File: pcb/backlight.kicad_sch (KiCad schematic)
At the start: 52 parts, among them U1 AL8860WT, U3 AL8860WT, U4 AL8860WT

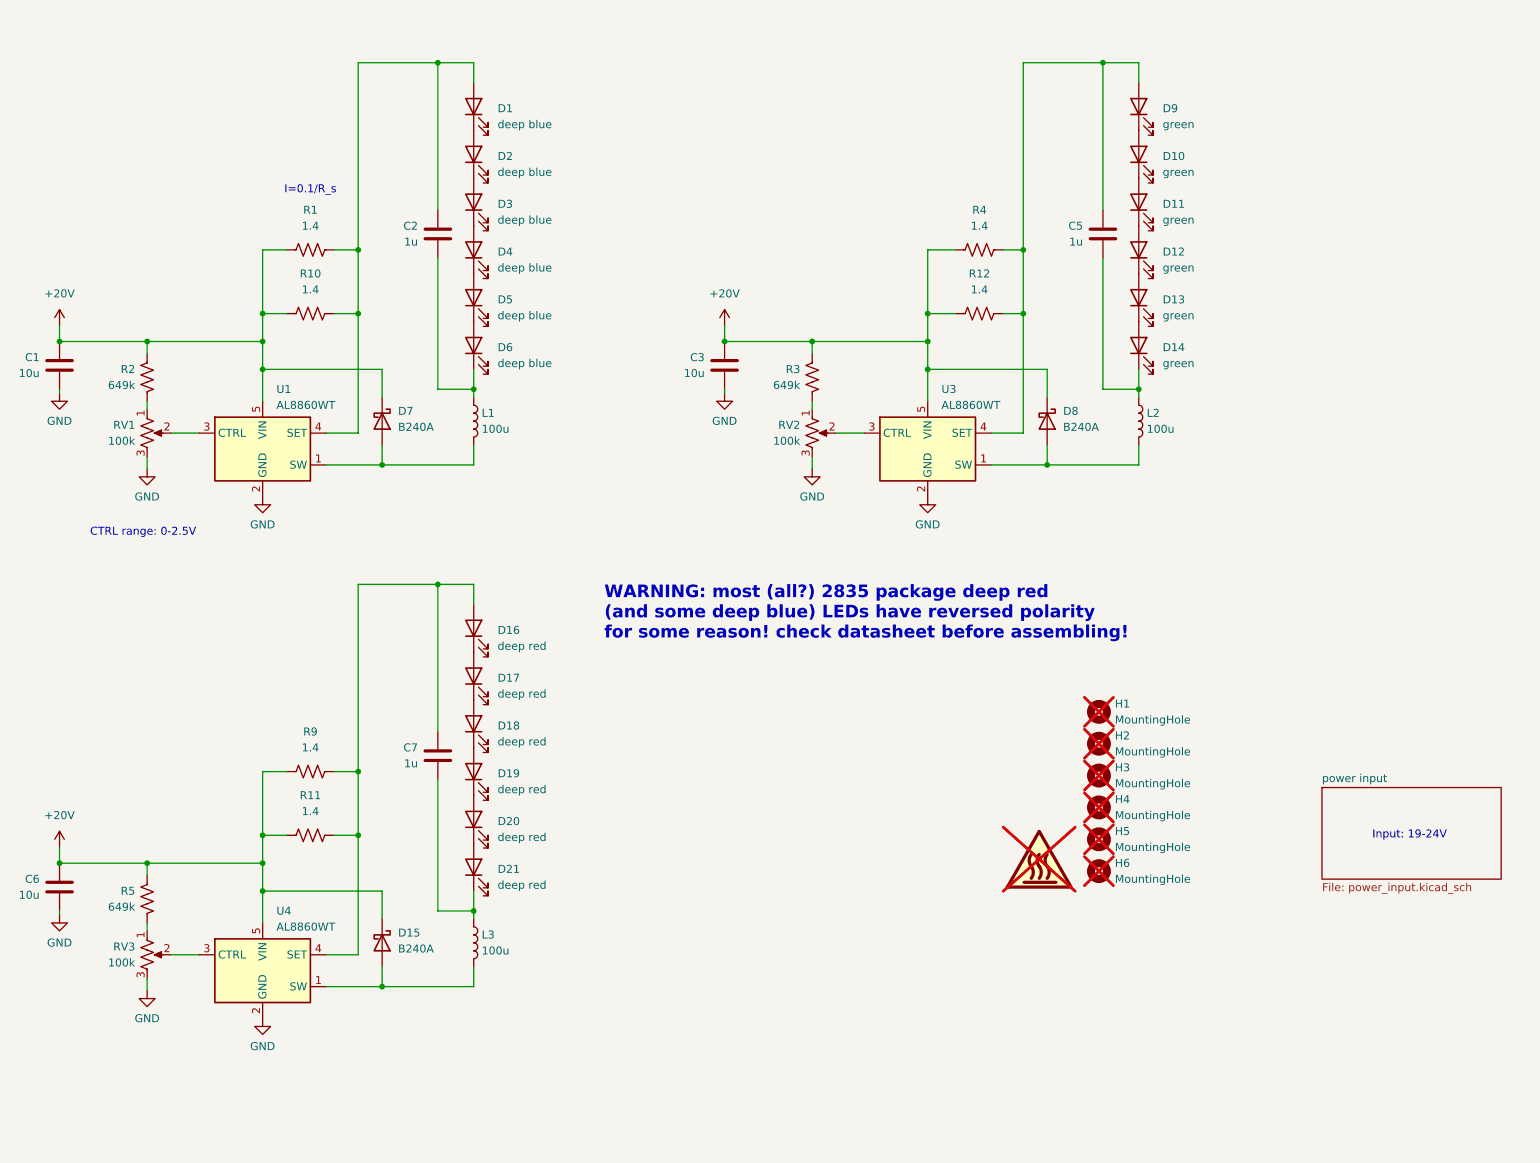
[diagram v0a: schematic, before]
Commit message: PCB for 4x5 scanlight
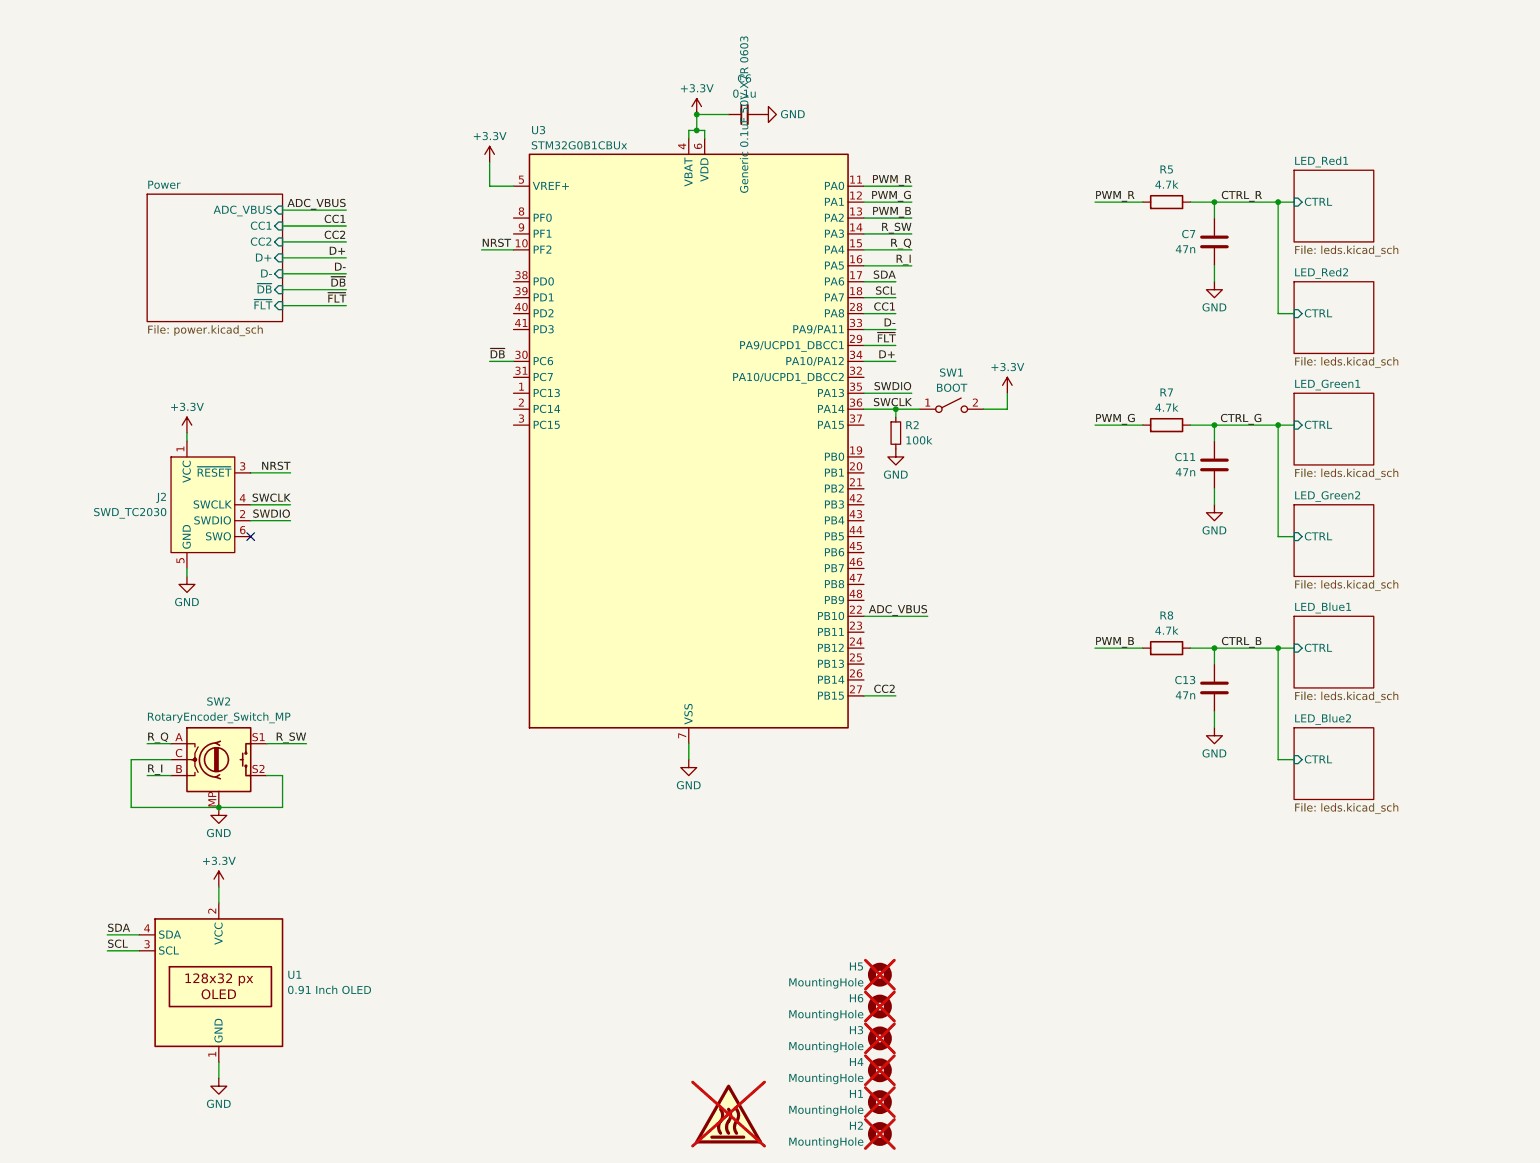
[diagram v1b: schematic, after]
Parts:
- removed C1, C3, C6: 10u, Capacitor_SMD:C_1210_3225Metric, symbol Device:C
- removed C2, C5: 1u, Capacitor_SMD:C_0603_1608Metric, symbol Device:C
- removed D1, D2, D3, D4, D5, D6: deep blue, LED_SMD:LED_PLCC_2835_Handsoldering, symbol Device:LED
- removed D10, D11, D12, D13, D14, D9: green, LED_SMD:LED_PLCC_2835_Handsoldering, symbol Device:LED
- removed D15, D7, D8: B240A, Diode_SMD:D_SMA, symbol Diode:MBRA340
- removed D16, D17, D18, D19, D20, D21: deep red, LED_SMD:LED_PLCC_2835_Handsoldering, symbol Device:LED
- removed L1, L2, L3: 100u, Inductor_SMD:L_Bourns_SRN8040TA, symbol Device:L
- removed R1, R10, R11, R12, R4, R9: 1.4, Resistor_SMD:R_1206_3216Metric, symbol Device:R_US
- removed R2, R3, R5: 649k, Resistor_SMD:R_0603_1608Metric, symbol Device:R_US
- removed RV1, RV2, RV3: 100k, Potentiometer_THT:Potentiometer_Bourns_PTV09A-1_Single_Vertical, symbol Device:R_Potentiometer_US
- removed U1, U3, U4: AL8860WT, Package_TO_SOT_SMD:TSOT-23-5, symbol Driver_LED:AL8860WT
- added C11, C13: 47n, Capacitor_SMD:C_0805_2012Metric, symbol Device:C
- added C6: 0.1u, Capacitor_SMD:C_0603_1608Metric, symbol Device:C_Small
- added J2: SWD_TC2030, Connector:Tag-Connect_TC2030-IDC-NL_2x03_P1.27mm_Vertical, symbol Connector:Conn_ARM_SWD_TagConnect_TC2030-NL
- added R2: 100k, Resistor_SMD:R_0603_1608Metric, symbol Device:R_Small
- added R5, R7, R8: 4.7k, Resistor_SMD:R_0603_1608Metric, symbol Device:R
- added SW1: BOOT, Jumper:SolderJumper-2_P1.3mm_Open_TrianglePad1.0x1.5mm, symbol Switch:SW_SPST
- added SW2: RotaryEncoder_Switch_MP, Rotary_Encoder:RotaryEncoder_Alps_EC11E-Switch_Vertical_H20mm, symbol Device:RotaryEncoder_Switch_MP
- added U1: 0.91 Inch OLED, Display:0.91_Inch_OLED, symbol Display_Graphic:0.91_Inch_OLED
- added U3: STM32G0B1CBUx, Package_DFN_QFN:QFN-48-1EP_7x7mm_P0.5mm_EP5.6x5.6mm, symbol MCU_ST_STM32G0:STM32G0B1CBUx
- C7: value 1u -> 47n; footprint Capacitor_SMD:C_0603_1608Metric -> Capacitor_SMD:C_0805_2012Metric; MPN Generic 1uF 25V 0603 X7R -> Generic 0.047uF 50V X7R 0805
- H1: renamed from H5; footprint Custom:MountingHole_2.2mm_M2_Mask_5mm -> MountingHole:MountingHole_2.2mm_M2_Mask_5mm; now left out of the parts list
- H2: renamed from H6; footprint Custom:MountingHole_2.2mm_M2_Mask_5mm -> MountingHole:MountingHole_2.2mm_M2_Mask_5mm; now left out of the parts list
- H3, H4: footprint Custom:MountingHole_2.2mm_M2_Mask_5mm -> MountingHole:MountingHole_2.2mm_M2_Mask_5mm; now left out of the parts list
- H5: renamed from H1; footprint Custom:MountingHole_2.2mm_M2_Mask_5mm -> MountingHole:MountingHole_2.2mm_M2_Mask_5mm; now left out of the parts list
- H6: renamed from H2; footprint Custom:MountingHole_2.2mm_M2_Mask_5mm -> MountingHole:MountingHole_2.2mm_M2_Mask_5mm; now left out of the parts list
- SYM1: renamed from SYM101; footprint Custom:hot-surface_1x -> Symbol:HOT; now left out of the parts list
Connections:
- net GND: now also C7.2, C11.2, C13.2, C6.2, J2.5 (GND), R2.2, SW2.C, SW2.MP, SW2.S2, U1.1 (GND), U3.49 (VSS), U3.7 (VSS)
- net CTRL_R: now reaches C7.1
- net CTRL_R: now also R5.1
- new net +3.3V: C6.1, J2.1 (VCC), SW1.2 (B), U1.2 (VCC), U3.4 (VBAT), U3.5 (VREF+), U3.6 (VDD)
- new net ADC_VBUS: U3.22 (PB10)
- new net CC1: U3.28 (PA8)
- new net CC2: U3.27 (PB15)
- new net CTRL_B: C13.1, R8.1
- new net CTRL_G: C11.1, R7.1
- new net D+: U3.34 (PA10/PA12)
- new net D-: U3.33 (PA9/PA11)
- new net NRST: J2.3 (~{RESET}), U3.10 (PF2)
- new net PWM_B: R8.2, U3.13 (PA2)
- new net PWM_G: R7.2, U3.12 (PA1)
- new net PWM_R: R5.2, U3.11 (PA0)
- new net R_I: SW2.B, U3.16 (PA5)
- new net R_Q: SW2.A, U3.15 (PA4)
- new net R_SW: SW2.S1, U3.14 (PA3)
- new net SCL: U1.3 (SCL), U3.18 (PA7)
- new net SDA: U1.4 (SDA), U3.17 (PA6)
- new net SWCLK: J2.4 (SWCLK), R2.1, SW1.1 (A), U3.36 (PA14)
- new net SWDIO: J2.2 (SWDIO), U3.35 (PA13)
- new net ~{DB}: U3.30 (PC6)
- new net ~{FLT}: U3.29 (PA9/UCPD1_DBCC1)
- no-connect marks 0 -> 1
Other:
- removed sheet power input
- added sheet LED_Blue1 (leds.kicad_sch)
- added sheet LED_Blue2 (leds.kicad_sch)
- added sheet LED_Green1 (leds.kicad_sch)
- added sheet LED_Green2 (leds.kicad_sch)
- added sheet LED_Red1 (leds.kicad_sch)
- added sheet LED_Red2 (leds.kicad_sch)
- added sheet Power (power.kicad_sch)
- note removed: "CTRL range: 0-2.5V"
- note removed: "I=0.1/R_s"
- note removed: "Input: 19-24V"
- note removed: "WARNING: most (all?) 2835 package deep red (and some deep blue) LEDs have reversed polarity for some reason! check datasheet before assembling!"
- moved on the sheet: H1, H2, H3, H4, H5, H6
